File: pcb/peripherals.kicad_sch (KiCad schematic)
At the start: 30 parts, among them J2 Conn_01x24_MountingPin, J3 Conn_02x10_Odd_Even, U4 TLV74328PDBVR, U5 NRF24L01_Breakout, U6 TLV74315PDBVR, U7 BMI270, U8 HYCW110-TF10-180B

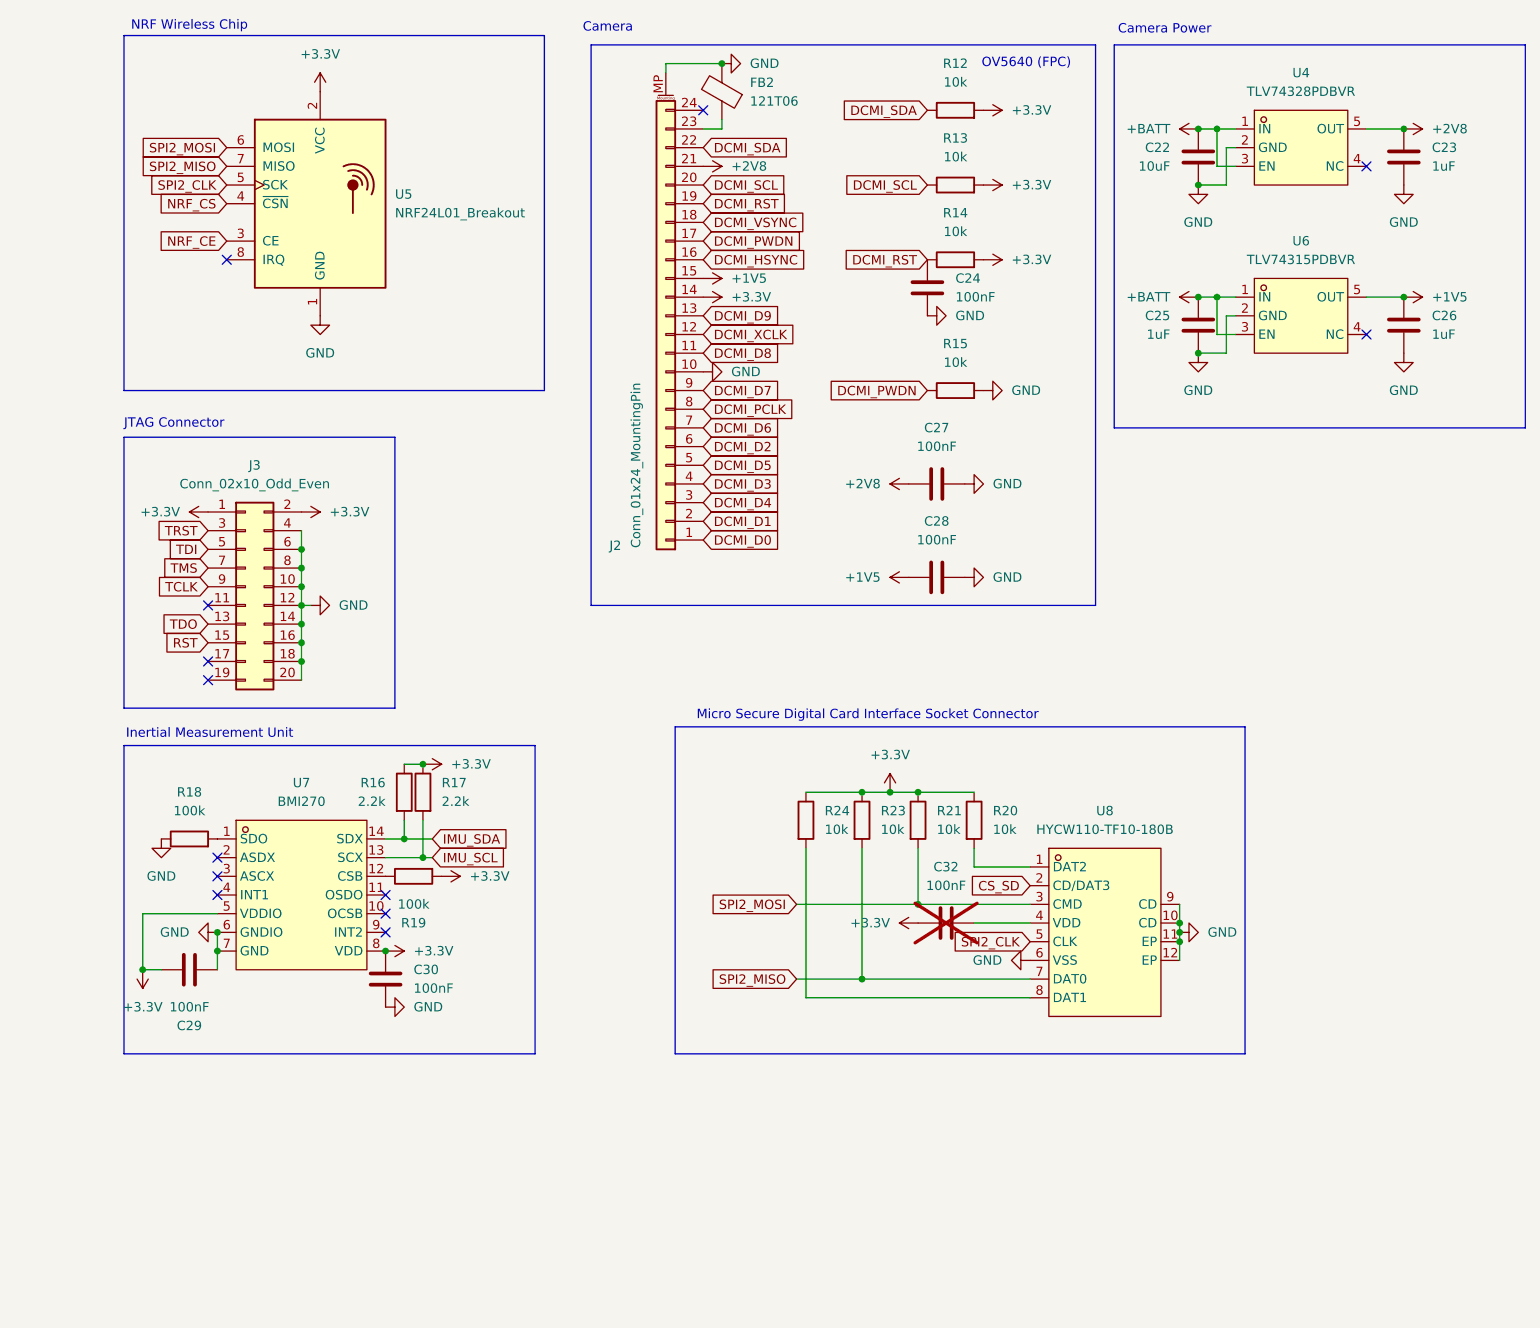
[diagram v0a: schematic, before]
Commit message: [pcb] invented the cutting edge, extremely innovative monke and ddg connectors
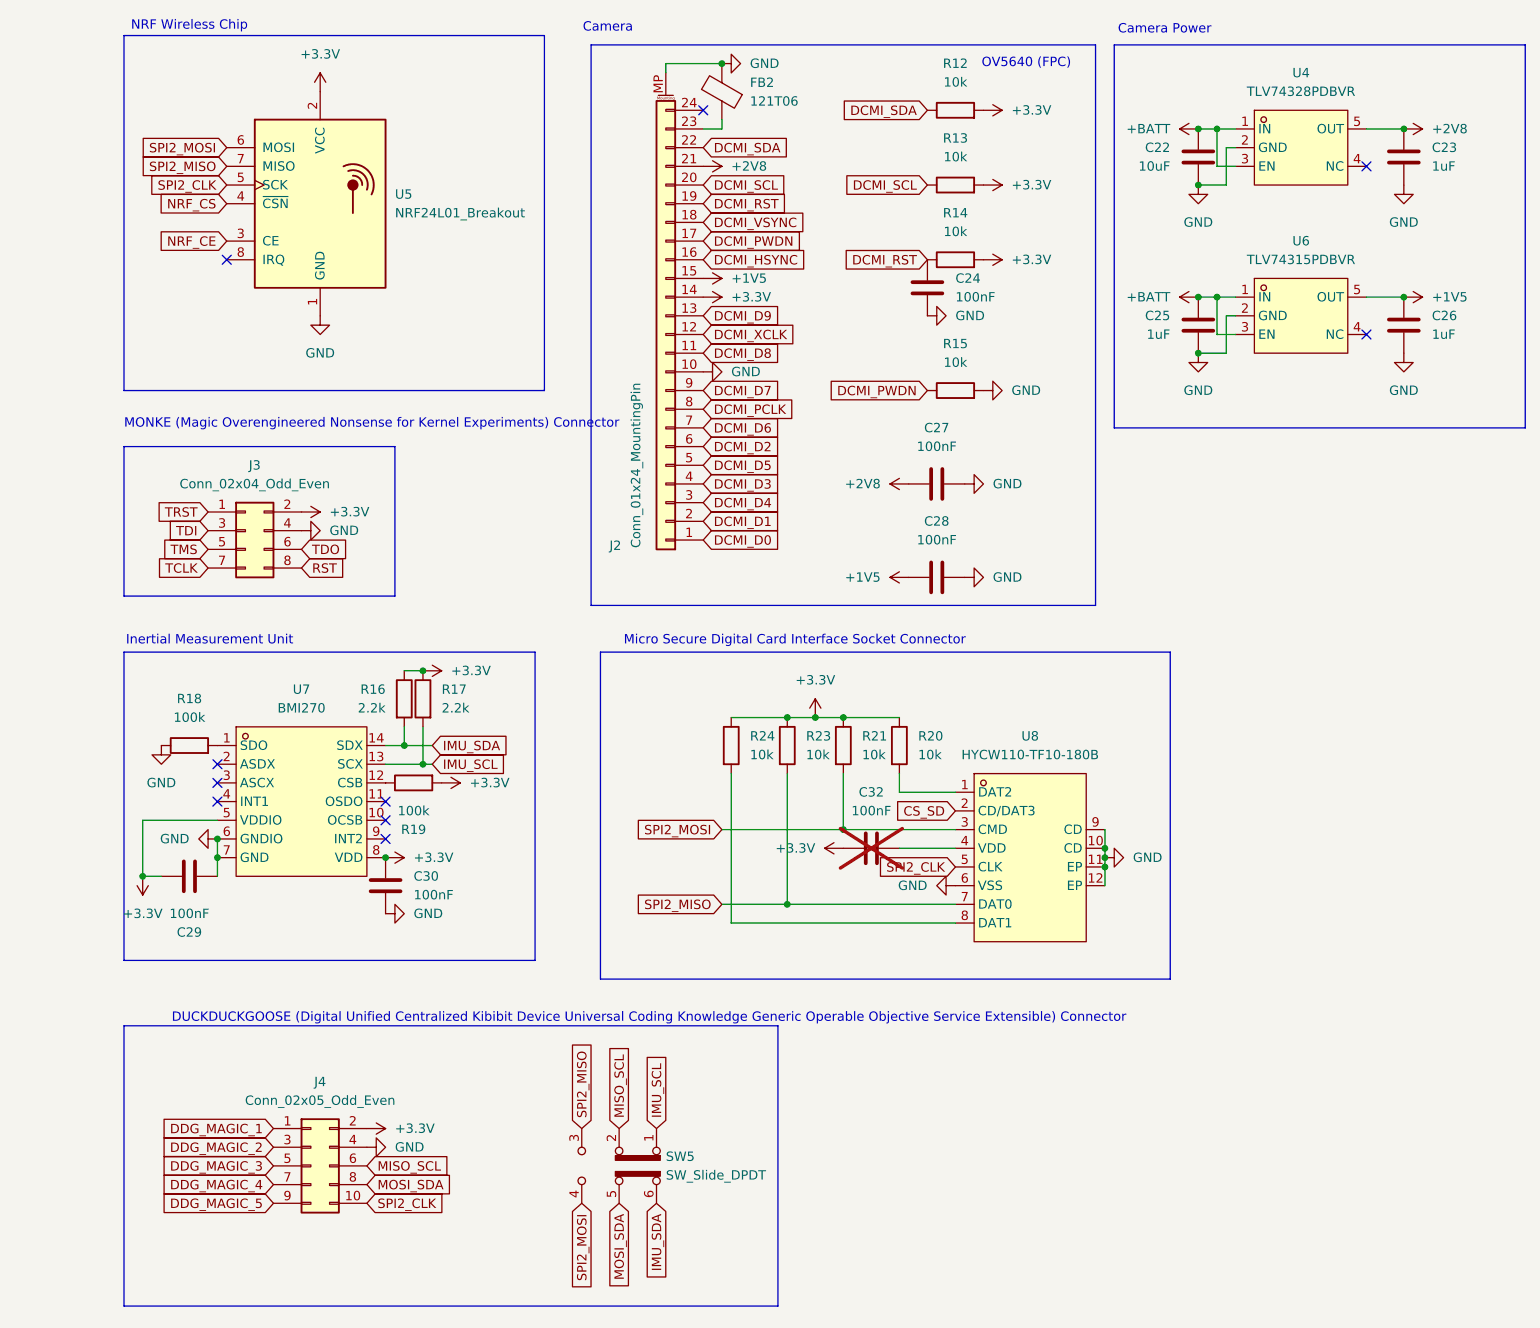
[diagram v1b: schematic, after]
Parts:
- removed J3: Conn_02x10_Odd_Even, Connector_PinHeader_2.54mm:PinHeader_2x10_P2.54mm_Vertical, symbol Connector_Generic:Conn_02x10_Odd_Even
- added J3: Conn_02x04_Odd_Even, symbol Connector_Generic:Conn_02x04_Odd_Even
- added J4: Conn_02x05_Odd_Even, symbol Connector_Generic:Conn_02x05_Odd_Even
- added SW5: SW_Slide_DPDT, symbol Switch:SW_Slide_DPDT
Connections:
- net +3.3V: now also J3.2 (Pin_2), J4.2 (Pin_2)
- net GND: now also J3.4 (Pin_4), J4.4 (Pin_4)
- net IMU_SCL: now also SW5.1 (A)
- net IMU_SDA: now also SW5.6 (C)
- net RST: now also J3.8 (Pin_8)
- net SPI2_CLK: now also J4.10 (Pin_10)
- net SPI2_MISO: now also SW5.3 (C)
- net SPI2_MOSI: now also SW5.4 (A)
- net TCLK: now also J3.7 (Pin_7)
- net TDI: now also J3.3 (Pin_3)
- net TDO: now also J3.6 (Pin_6)
- net TMS: now also J3.5 (Pin_5)
- net TRST: now also J3.1 (Pin_1)
- new net DDG_MAGIC_1: J4.1 (Pin_1)
- new net DDG_MAGIC_2: J4.3 (Pin_3)
- new net DDG_MAGIC_3: J4.5 (Pin_5)
- new net DDG_MAGIC_4: J4.7 (Pin_7)
- new net DDG_MAGIC_5: J4.9 (Pin_9)
- new net MISO_SCL: J4.6 (Pin_6), SW5.2 (B)
- new net MOSI_SDA: J4.8 (Pin_8), SW5.5 (B)
- no-connect marks 13 -> 10
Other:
- note added: "DUCKDUCKGOOSE (Digital Unified Centralized Kibibit Device Universal Coding Knowledge Generic Operable Objective Service Extensible) Connector"
- note added: "MONKE (Magic Overengineered Nonsense for Kernel Experiments) Connector"
- note removed: "JTAG Connector"
- moved on the sheet: C29, C30, C32, R16, R17, R18, R19, R20, R21, R23, R24, U7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
